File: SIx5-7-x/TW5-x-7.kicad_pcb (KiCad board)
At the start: 2 copper layers, 31 x 53 mm, 4 parts

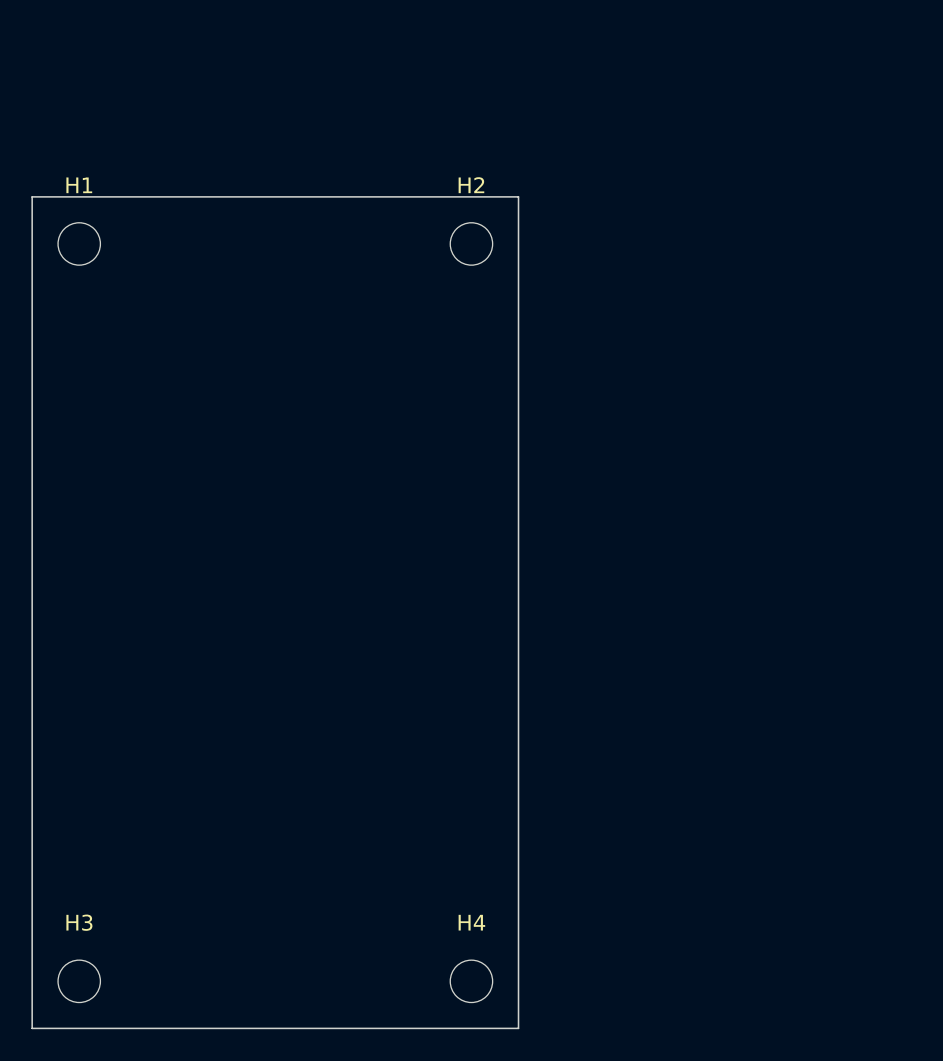
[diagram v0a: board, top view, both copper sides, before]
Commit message: テンプレを作成↓
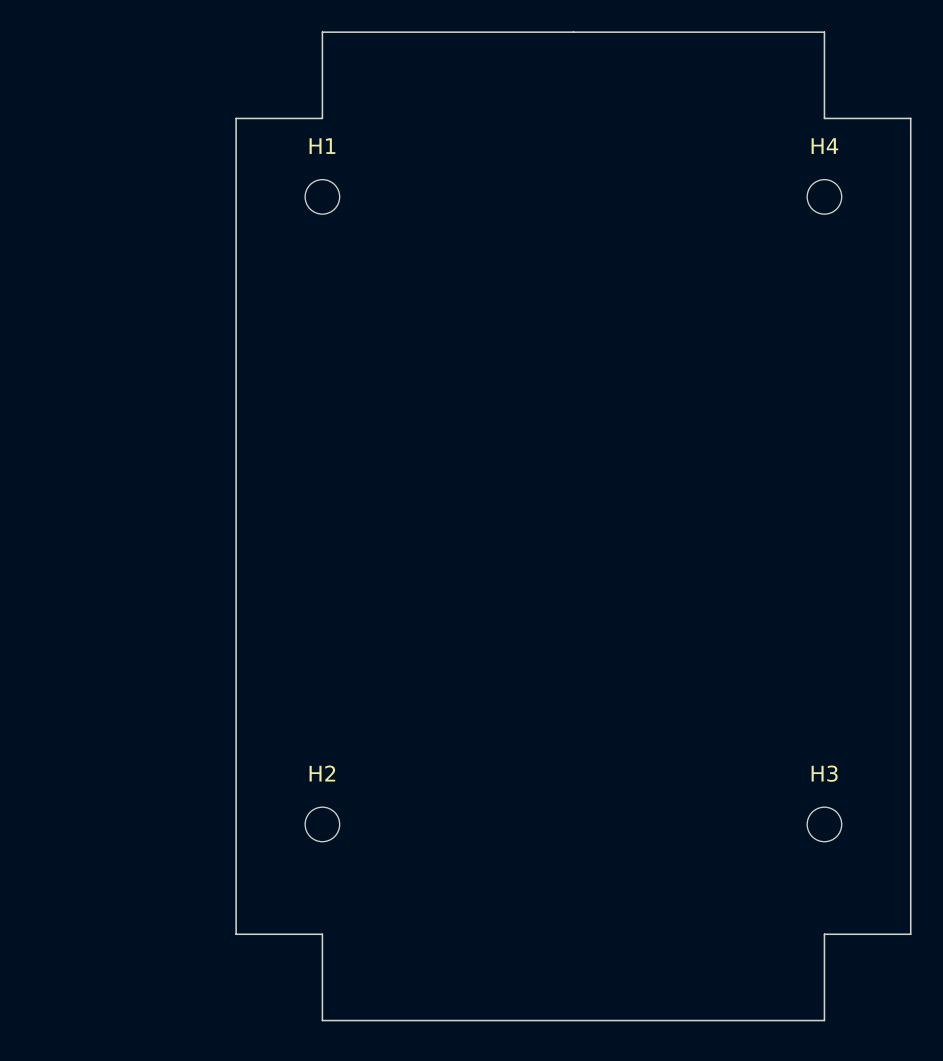
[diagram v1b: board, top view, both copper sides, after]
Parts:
- H1, H2, H3, H4: footprint MountingHole:MountingHole_2.7mm -> MountingHole:MountingHole_2.2mm_M2
- moved H4 54.8 mm to (176.0, 80.0)
- moved H3 48.5 mm to (176.0, 120.0)
- moved H2 38.2 mm to (144.0, 120.0)
- moved H1 15.8 mm to (144.0, 80.0)
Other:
- board size 31 x 53 mm -> 43 x 63 mm
